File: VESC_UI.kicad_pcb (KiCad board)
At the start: 2 copper layers, 85 x 56 mm, 43 parts, among them K1 K_0051, K6 K_0038, Q1 Q_0010, Q2 Q_0010, SW1 EC12D1564402, U1 U_0076

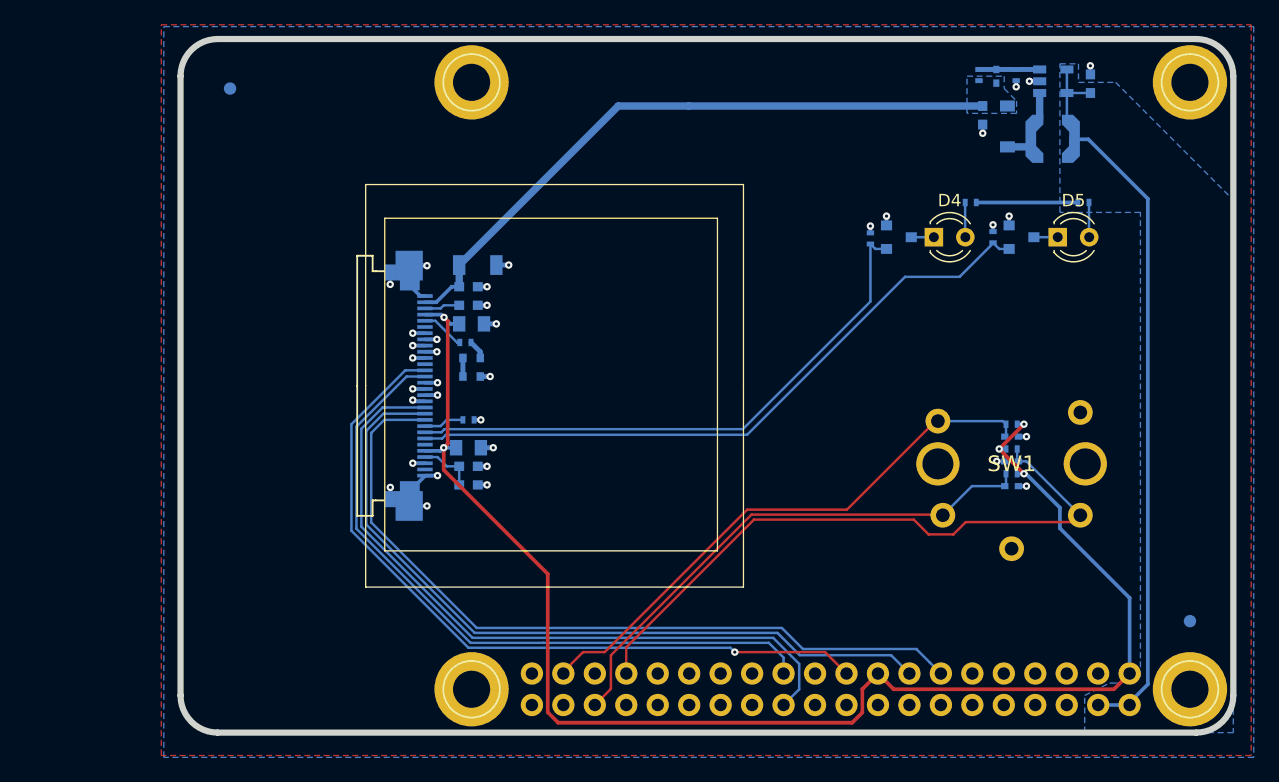
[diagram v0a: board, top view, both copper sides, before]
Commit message: first finished version
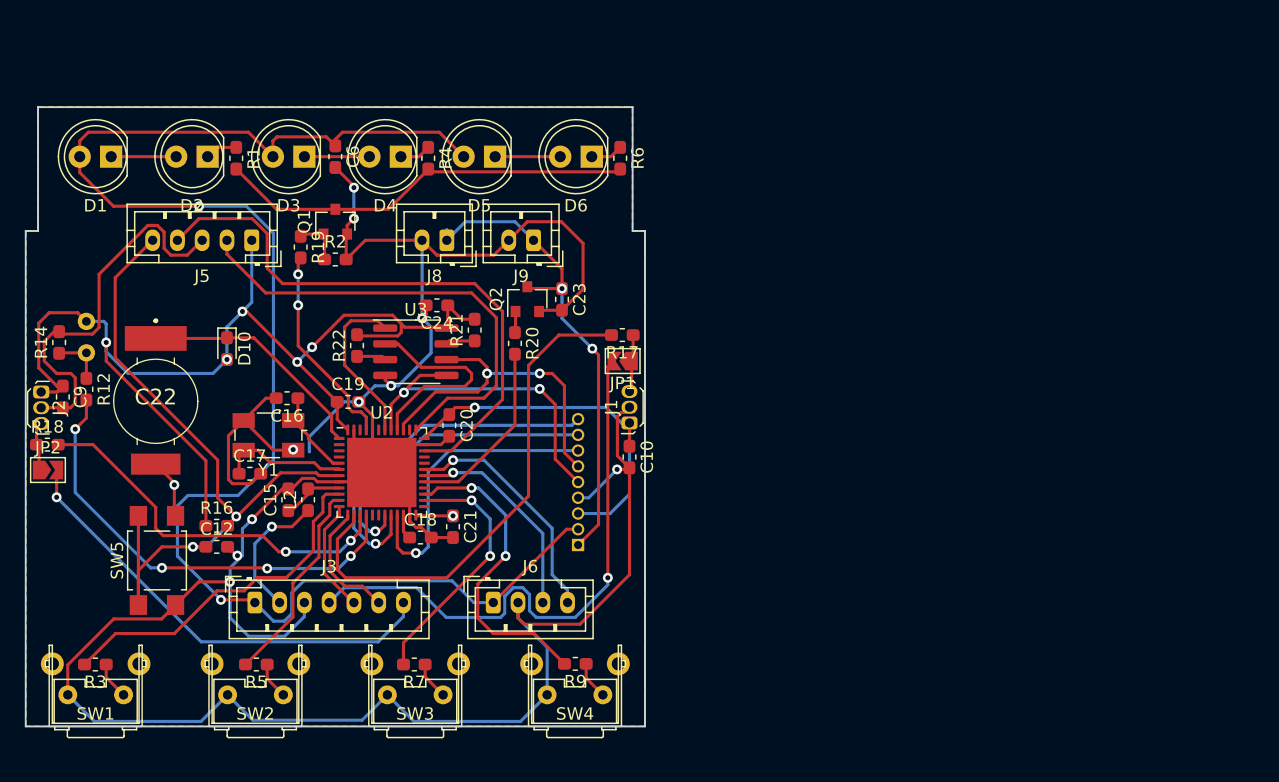
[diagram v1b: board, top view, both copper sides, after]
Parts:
- removed C1: C_0003, DVB_Capacitors_Ceramic:C_0603
- removed C13, C14: C_0002, DVB_Capacitors_Ceramic:C_0402
- removed C2: C_0013, DVB_Capacitors_Ceramic:C_0402
- removed C3: C_0033, DVB_Capacitors_Ceramic:C_0603
- removed C4: C_0036, DVB_Capacitors_Ceramic:C_0603
- removed C5: C_0041, DVB_Capacitors_Ceramic:C_1206
- removed C7, C8: C_0056, DVB_Capacitors_Ceramic:C_0805
- removed K1: K_0051, DVB_Displays:OLED128x128-1P5
- removed K6: K_0038, DVB_Connectors:SSQ-120-03-G-D
- removed L1: L_0011, DVB_Inductors:L_4018-Coilcraft
- removed R10, R11: R_0020, DVB_Resistors:R_0402
- removed R8: R_0053, DVB_Resistors:R_0402
- removed REF** (x2): CircleWhite1mm, DVB_Fiducials:REF_1mm
- removed REF** (x4): VAL**, DVB_Mechanicals:1pin
- removed REF**: VAL**, DVB_Mechanicals:DVBLOGO
- removed U1: U_0076, DVB_SOT:SOT_23-5
- added C12: C_0033, Capacitor_SMD:C_0603_1608Metric_Pad1.05x0.95mm_HandSolder, F.Cu at (129.4, 110.5)
- added C16: C_Small, Capacitor_SMD:C_0603_1608Metric_Pad1.05x0.95mm_HandSolder, F.Cu at (135.1, 98.5)
- added C17: C_Small, Capacitor_SMD:C_0603_1608Metric_Pad1.05x0.95mm_HandSolder, F.Cu at (132.1, 104.6)
- added C18: 4.7u, Capacitor_SMD:C_0603_1608Metric_Pad1.05x0.95mm_HandSolder, F.Cu at (145.9, 109.8)
- added C19: C_Small, Capacitor_SMD:C_0603_1608Metric_Pad1.05x0.95mm_HandSolder, F.Cu at (140.0, 98.8)
- added C20: C_Small, Capacitor_SMD:C_0603_1608Metric_Pad1.05x0.95mm_HandSolder, F.Cu at (148.2, 100.7)
- added C21: C_Small, Capacitor_SMD:C_0603_1608Metric_Pad1.05x0.95mm_HandSolder, F.Cu at (148.5, 108.9)
- added C22: CP_Small, SamacSys_Parts:DSK3R3H334THL, F.Cu at (124.5, 98.8)
- added C23: C_0033, Capacitor_SMD:C_0603_1608Metric_Pad1.05x0.95mm_HandSolder, F.Cu at (157.3, 90.5)
- added C24: C_0033, Capacitor_SMD:C_0603_1608Metric_Pad1.05x0.95mm_HandSolder, F.Cu at (147.2, 91.0)
- added D10: D_Schottky_Small_ALT, Diode_SMD:D_0603_1608Metric_Pad1.05x0.95mm_HandSolder, F.Cu at (130.2, 94.5)
- added D6: LED_Small_ALT, LED_THT:LED_D5.0mm_Clear, F.Cu at (159.7, 79.0)
- added J1: Hall_SS443A, Package_TO_SOT_THT:TO-92Flat, F.Cu at (162.8, 100.5)
- added J2: Hall_SS443A, Package_TO_SOT_THT:TO-92Flat, F.Cu at (115.2, 98.0)
- added J3: Conn_01x07_Male, Connector_JST:JST_PH_B7B-PH-K_1x07_P2.00mm_Vertical, F.Cu at (132.5, 115.0)
- added J4: Conn_01x09_Female, Connector_PinHeader_1.27mm:PinHeader_1x09_P1.27mm_Vertical, B.Cu at (158.6, 110.3)
- added J5: Conn_01x05_Male, Connector_JST:JST_PH_B5B-PH-K_1x05_P2.00mm_Vertical, F.Cu at (132.2, 85.8)
- added J6: Conn_01x04_Male, Connector_JST:JST_PH_B4B-PH-K_1x04_P2.00mm_Vertical, F.Cu at (151.8, 115.0)
- added J8: Conn_01x02_Male, Connector_JST:JST_PH_B2B-PH-K_1x02_P2.00mm_Vertical, F.Cu at (148.0, 85.8)
- added J9: Conn_01x02_Male, Connector_JST:JST_PH_B2B-PH-K_1x02_P2.00mm_Vertical, F.Cu at (155.0, 85.8)
- added JP1: Jumper_NC_Small, Jumper:SolderJumper-2_P1.3mm_Open_TrianglePad1.0x1.5mm, F.Cu at (162.2, 95.5)
- added JP2: Jumper_NC_Small, Jumper:SolderJumper-2_P1.3mm_Open_TrianglePad1.0x1.5mm, F.Cu at (115.8, 104.3)
- added L2: MMZ1608B121C, Inductor_SMD:L_0603_1608Metric_Pad1.05x0.95mm_HandSolder, F.Cu at (136.8, 106.7)
- added R12: R_Small, Resistor_SMD:R_0603_1608Metric_Pad1.05x0.95mm_HandSolder, F.Cu at (118.9, 97.8)
- added R13: R_PHOTO, Resistor_THT:R_Axial_DIN0204_L3.6mm_D1.6mm_P2.54mm_Vertical, B.Cu at (118.9, 92.3)
- added R14: R_0020, Resistor_SMD:R_0603_1608Metric_Pad1.05x0.95mm_HandSolder, F.Cu at (116.7, 94.0)
- added R16: R_Small, Resistor_SMD:R_0603_1608Metric_Pad1.05x0.95mm_HandSolder, F.Cu at (129.4, 108.8)
- added R17: R_Small, Resistor_SMD:R_0603_1608Metric_Pad1.05x0.95mm_HandSolder, F.Cu at (162.2, 93.4)
- added R18: R_Small, Resistor_SMD:R_0603_1608Metric_Pad1.05x0.95mm_HandSolder, F.Cu at (115.8, 102.2)
- added R19: R_0020, Resistor_SMD:R_0603_1608Metric_Pad1.05x0.95mm_HandSolder, F.Cu at (136.2, 86.3)
- added R20: R_0020, Resistor_SMD:R_0603_1608Metric_Pad1.05x0.95mm_HandSolder, F.Cu at (153.5, 94.1)
- added R21: R_Small, Resistor_SMD:R_0603_1608Metric_Pad1.05x0.95mm_HandSolder, F.Cu at (150.2, 93.0)
- added R22: R_Small, Resistor_SMD:R_0603_1608Metric_Pad1.05x0.95mm_HandSolder, F.Cu at (140.8, 94.2)
- added SW2: SW_Push, SamacSys_Parts:Vertical_push_button, F.Cu at (132.6, 121.2)
- added SW3: SW_Push, SamacSys_Parts:Vertical_push_button, F.Cu at (145.4, 121.2)
- added SW4: SW_Push, SamacSys_Parts:Vertical_push_button, F.Cu at (158.3, 121.2)
- added SW5: SW_Push, Button_Switch_SMD:SW_SPST_TL3305A, F.Cu at (124.6, 111.6)
- added U2: STM32F401CEUx, Package_DFN_QFN:QFN-48-1EP_7x7mm_P0.5mm_EP5.6x5.6mm, F.Cu at (142.8, 104.5)
- added U3: M95M04-DR, Package_SO:SOIC-8_3.9x4.9mm_P1.27mm, F.Cu at (145.5, 94.8)
- added Y1: Crystal_GND24_Small, Crystal:Crystal_SMD_Abracon_ABM3B-4Pin_5.0x3.2mm, F.Cu at (133.6, 101.5)
- C10, C6: value C_0036 -> C_Small; footprint DVB_Capacitors_Ceramic:C_0603 -> Capacitor_SMD:C_0603_1608Metric_Pad1.05x0.95mm_HandSolder; moved to F.Cu
- C15: value C_0002 -> C_0033; footprint DVB_Capacitors_Ceramic:C_0402 -> Capacitor_SMD:C_0603_1608Metric_Pad1.05x0.95mm_HandSolder; moved to F.Cu
- C9: value C_0033 -> C_Small; footprint DVB_Capacitors_Ceramic:C_0603 -> Capacitor_SMD:C_0603_1608Metric_Pad1.05x0.95mm_HandSolder; moved to F.Cu
- D1: value D_0021 -> LED_Small_ALT; footprint DVB_Diodes:D_SOD-123 -> LED_THT:LED_D5.0mm_Clear; moved to F.Cu
- D2, D3: value D_0022 -> LED_Small_ALT; footprint DVB_Diodes:D_SOD-523 -> LED_THT:LED_D5.0mm_Clear; moved to F.Cu
- D4: value D_0040 -> LED_Small_ALT; footprint Lib_KiCount_Footprint:LED_D3.0mm_FlatTop-Green -> LED_THT:LED_D5.0mm_Clear
- D5: value D_0039 -> LED_Small_ALT; footprint Lib_KiCount_Footprint:LED_D3.0mm_FlatTop-Red -> LED_THT:LED_D5.0mm_Clear
- Q1, Q2: value Q_0010 -> Q_0010-DVB_Q; footprint DVB_SOT:SOT_23 -> Package_TO_SOT_SMD:SOT-23; moved to F.Cu
- R1: value R_0107 -> R_0020; footprint DVB_Resistors:R_0402 -> Resistor_SMD:R_0603_1608Metric_Pad1.05x0.95mm_HandSolder; moved to F.Cu
- R2: value R_0108 -> R_0020; footprint DVB_Resistors:R_0402 -> Resistor_SMD:R_0603_1608Metric_Pad1.05x0.95mm_HandSolder; moved to F.Cu
- R3: value R_0110 -> R_Small; footprint DVB_Resistors:R_0402 -> Resistor_SMD:R_0603_1608Metric_Pad1.05x0.95mm_HandSolder; moved to F.Cu
- R4: value R_0019 -> R_0020; footprint DVB_Resistors:R_0402 -> Resistor_SMD:R_0603_1608Metric_Pad1.05x0.95mm_HandSolder; moved to F.Cu
- R5, R9: value R_0020 -> R_Small; footprint DVB_Resistors:R_0402 -> Resistor_SMD:R_0603_1608Metric_Pad1.05x0.95mm_HandSolder; moved to F.Cu
- R6: footprint DVB_Resistors:R_0402 -> Resistor_SMD:R_0603_1608Metric_Pad1.05x0.95mm_HandSolder; moved to F.Cu
- R7: value R_0053 -> R_Small; footprint DVB_Resistors:R_0402 -> Resistor_SMD:R_0603_1608Metric_Pad1.05x0.95mm_HandSolder; moved to F.Cu
- SW1: value EC12D1564402 -> SW_Push; footprint Lib_KiCount_Footprint:EC12D1564402 -> SamacSys_Parts:Vertical_push_button
- moved SW1 76.0 mm to (119.7, 121.2), turned to 0 degrees
- moved D1 72.4 mm to (120.9, 79.0), turned to 180 degrees
- moved R5 68.8 mm to (132.6, 120.0), turned to 180 degrees
- moved R7 65.7 mm to (145.4, 120.0), turned to 180 degrees
- moved R1 60.3 mm to (131.0, 79.1), turned to 270 degrees
- moved C15 58.6 mm to (135.2, 106.7), turned to 90 degrees
- moved R2 56.9 mm to (139.0, 87.3), turned to 0 degrees
- moved D5 47.2 mm to (151.9, 79.0), turned to 180 degrees
- moved Q1 45.5 mm to (139.0, 84.2), turned to 90 degrees
- moved D4 44.8 mm to (144.3, 79.0), turned to 180 degrees
- moved R9 41.8 mm to (158.4, 120.0), turned to 180 degrees
- moved Q2 40.2 mm to (154.5, 90.5), turned to 90 degrees
- moved R3 39.6 mm to (119.6, 120.0), turned to 180 degrees
- moved R6 38.2 mm to (162.0, 79.1), turned to 270 degrees
- moved C9 33.2 mm to (117.0, 98.4), turned to 270 degrees
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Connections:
- C10 pad 1: Net-(C10-Pad1) -> +3V3
- C15 pad 1: GND -> /VREF+
- C15 pad 2: Button3 -> GND
- C6 pad 1: Net-(C6-Pad1) -> +5V
- C9 pad 1: GND -> +3V3
- C9 pad 2: Net-(C10-Pad1) -> GND
- D1 pad 1: +12V -> Net-(D1-Pad1)
- D1 pad 2: Net-(D1-Pad2) -> +5V
- D2 pad 2: Net-(D2-Pad2) -> Net-(D1-Pad1)
- D3 pad 1: GND -> Net-(D3-Pad1)
- D3 pad 2: Net-(D2-Pad1) -> +5V
- D4 pad 2: Net-(D4-Pad2) -> Net-(D3-Pad1)
- D5 pad 2: Net-(D5-Pad2) -> +5V
- Q1 pad 1: /GREEN_LED -> Net-(Q1-Pad1)
- Q1 pad 3: Net-(D4-Pad1) -> Net-(Q1-Pad3)
- Q2 pad 1: /RED_LED -> Net-(Q2-Pad1)
- Q2 pad 3: Net-(D5-Pad1) -> +12V
- R1 pad 1: +12V -> Net-(D2-Pad1)
- R1 pad 2: Net-(C2-Pad2) -> Net-(Q1-Pad3)
- R2 pad 1: Net-(C2-Pad2) -> Net-(Q1-Pad1)
- R3 pad 1: Net-(K1-Pad5) -> Net-(R3-Pad1)
- R3 pad 2: Net-(D2-Pad2) -> /BUTTON_1
- R4 pad 1: GND -> Net-(D4-Pad1)
- R4 pad 2: Net-(K1-Pad22) -> Net-(Q1-Pad3)
- R5 pad 1: /RED_LED -> Net-(R5-Pad1)
- R5 pad 2: GND -> /BUTTON_2
- R6 pad 1: +3.3V -> Net-(D6-Pad1)
- R6 pad 2: Button3 -> Net-(Q1-Pad3)
- R7 pad 1: +5V -> Net-(R7-Pad1)
- R7 pad 2: Net-(D5-Pad2) -> /BUTTON_3
- R9 pad 1: /GREEN_LED -> Net-(R9-Pad1)
- R9 pad 2: GND -> /BUTTON_4
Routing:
- net GND: track 37.1 -> 277.8 mm, vias 35 -> 11
- net +3V3: track 0.00 -> 137.2 mm, vias 0 -> 8
- net +3.3V: track 119.5 -> 0.00 mm, vias 5 -> 0
- net SPI_RES: track 63.1 -> 0.00 mm
- net SPI_DC: track 61.7 -> 0.00 mm
- net SPI_MOSI: track 61.1 -> 0.00 mm, vias 1 -> 0
- net /NRST: track 0.00 -> 59.3 mm, vias 0 -> 2
- net SPI_CS: track 57.5 -> 0.00 mm
- net SPI_SCK: track 55.5 -> 0.00 mm
- net +5V: track 71.8 -> 127.3 mm, vias 0 -> 2
- net /RED_LED: track 53.6 -> 0.00 mm
- net Button2: track 52.0 -> 0.00 mm
- net /Accelerator: track 0.00 -> 46.9 mm, vias 0 -> 1
- net /SWDIO: track 0.00 -> 46.8 mm
- net /GREEN_LED: track 46.4 -> 0.00 mm
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- added copper zone on B.Cu, net (none)
- added copper zone on In2.Cu_+3.3, net +3V3
- added copper zone on In1.Cu_GND, net GND
- removed copper zone on B.Cu, net +12V
- removed copper zone on B.Cu, net +5V
- removed copper zone on B.Cu, net GND
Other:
- board size 85 x 56 mm -> 50 x 50 mm
- copper layers 2 -> 4
- net class Default: trace_width 0.2 -> 0.25; via_dia 0.6 -> 0.8; via_drill 0.25 -> 0.4
- net class Power removed
- net class VPORTP removed
- net class power added: clearance 0.4, trace_width 0.6, via_dia 0.8, via_drill 0.4
- rule trace_min: 0.15 -> 0.2
- rule via_min_drill: 0.25 -> 0.3
- board text removed: "MTR GUI PI v1.1.0"
